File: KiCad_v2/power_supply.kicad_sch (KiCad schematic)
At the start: 32 parts, among them U1 LT8582EDKD-PBF, U6 MCP73871, U7 LM3940IMP-3.3

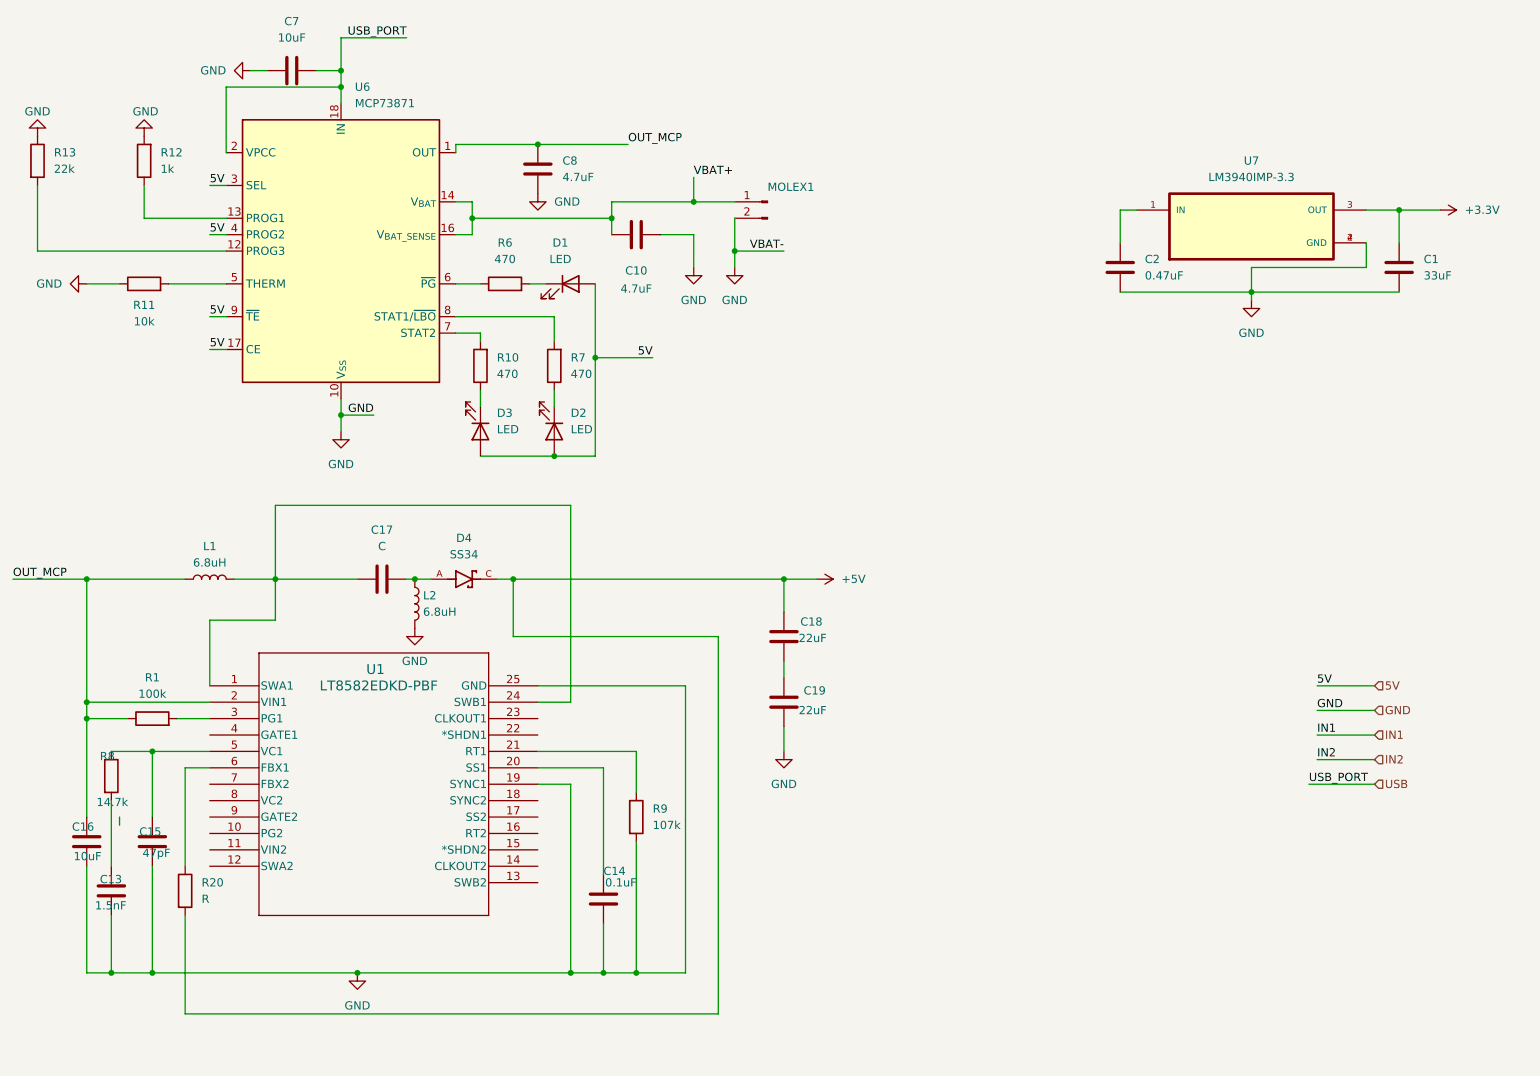
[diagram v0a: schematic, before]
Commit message: circuito terminado de LT8582, falta calcular valores
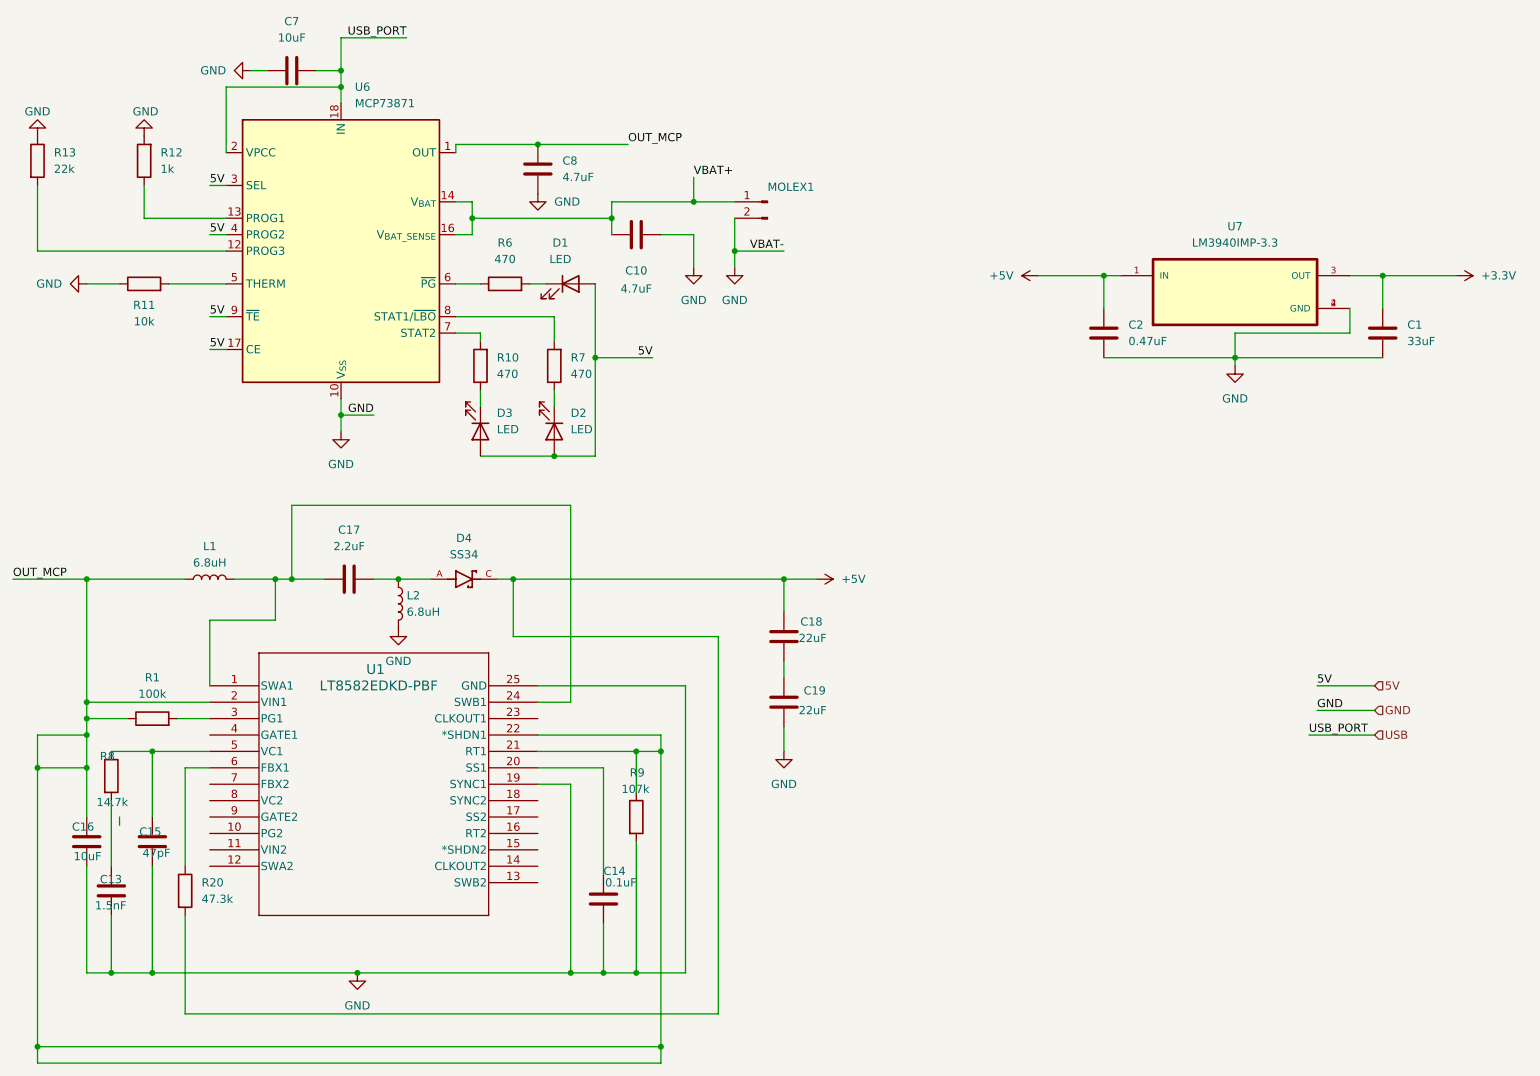
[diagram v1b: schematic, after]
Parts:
- C17: value C -> 2.2uF
- R20: value R -> 47.3k
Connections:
- net +5V: now also C2.1, U7.1 (IN)
- net OUT_MCP: now also R9.1, U1.21 (RT1), U1.22 (*SHDN1)
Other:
- moved on the sheet: C1, C17, C2, L2, U7
